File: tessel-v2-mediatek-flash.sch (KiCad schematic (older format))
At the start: 2 parts

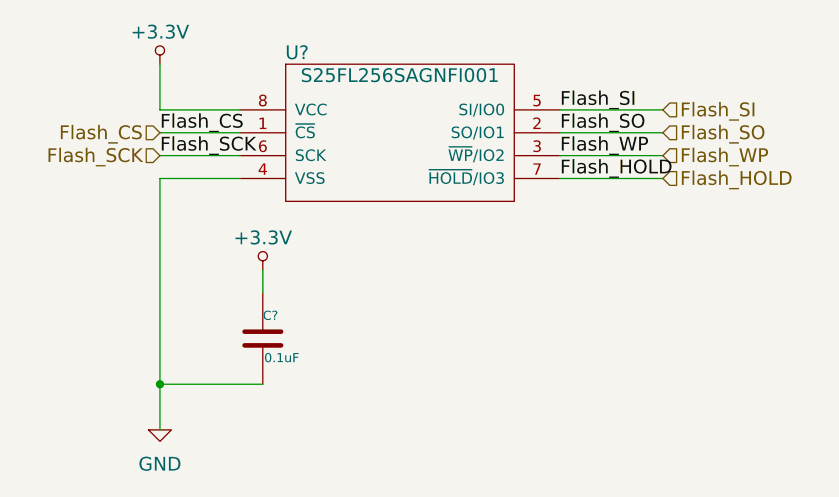
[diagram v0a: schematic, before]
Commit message: annotated
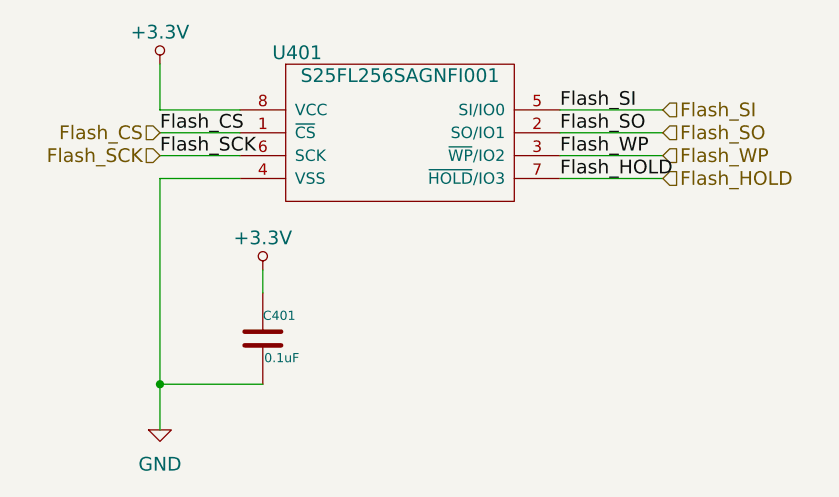
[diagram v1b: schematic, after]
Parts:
- gave numbers to parts that had none: 2
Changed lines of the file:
@@
 $EndDescr
 $Comp
-L S25FL256SAGNFI001 U?
+L S25FL256SAGNFI001 U401
 U 1 1 548FCC1A
 P 7800 4350
-F 0 "U?" H 7350 4700 60  0000 C CNN
+F 0 "U401" H 7350 4700 60  0000 C CNN
 F 1 "S25FL256SAGNFI001" H 7800 4600 60  0000 C CNN
 F 2 "" H 7400 5350 60  0000 C CNN
@@
 Flash_SCK
 $Comp
-L GND #PWR?
+L GND #PWR402
 U 1 1 548FCCD4
 P 6750 5650
-F 0 "#PWR?" H 6750 5400 60  0001 C CNN
+F 0 "#PWR402" H 6750 5400 60  0001 C CNN
 F 1 "GND" H 6750 5500 60  0000 C CNN
 F 2 "" H 6750 5650 60  0000 C CNN
@@
 	6750 4550 6750 5650
 $Comp
-L +3.3V #PWR?
+L +3.3V #PWR401
 U 1 1 548FCD0C
 P 6750 4050
-F 0 "#PWR?" H 6750 3900 60  0001 C CNN
+F 0 "#PWR401" H 6750 3900 60  0001 C CNN
 F 1 "+3.3V" H 6750 4190 60  0000 C CNN
 F 2 "" H 6750 4050 60  0000 C CNN
@@
 	6750 4250 6750 4050
 $Comp
-L C C?
+L C C401
 U 1 1 548FCD34
 P 7200 5250
-F 0 "C?" H 7200 5350 40  0000 L CNN
+F 0 "C401" H 7200 5350 40  0000 L CNN
 F 1 "0.1uF" H 7206 5165 40  0000 L CNN
 F 2 "" H 7238 5100 30  0000 C CNN
@@
 Connection ~ 6750 5450
 $Comp
-L +3.3V #PWR?
+L +3.3V #PWR403
 U 1 1 548FCD90
 P 7200 4950
-F 0 "#PWR?" H 7200 4800 60  0001 C CNN
+F 0 "#PWR403" H 7200 4800 60  0001 C CNN
 F 1 "+3.3V" H 7200 5090 60  0000 C CNN
 F 2 "" H 7200 4950 60  0000 C CNN

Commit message: give nF some love
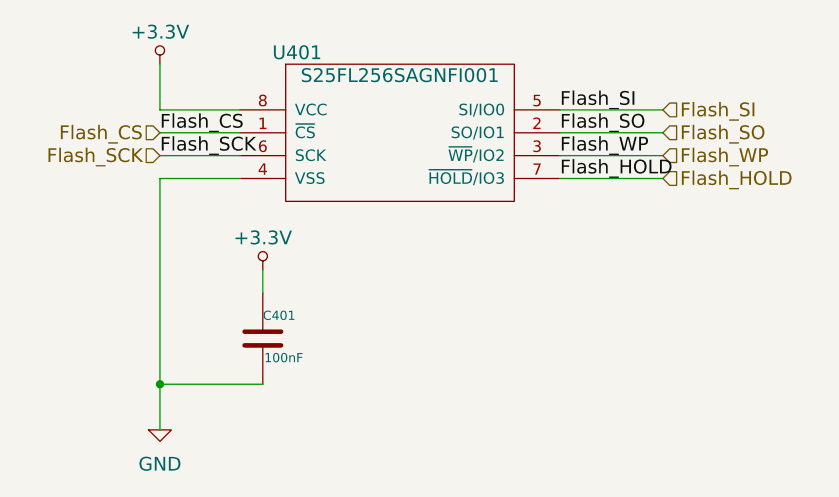
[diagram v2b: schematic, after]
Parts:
- C401: value 0.1uF -> 100nF
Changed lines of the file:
@@
 P 7200 5250
 F 0 "C401" H 7200 5350 40  0000 L CNN
-F 1 "0.1uF" H 7206 5165 40  0000 L CNN
+F 1 "100nF" H 7206 5165 40  0000 L CNN
 F 2 "" H 7238 5100 30  0000 C CNN
 F 3 "" H 7200 5250 60  0000 C CNN
